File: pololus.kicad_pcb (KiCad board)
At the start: 2 copper layers, 50 x 50 mm, 9 parts

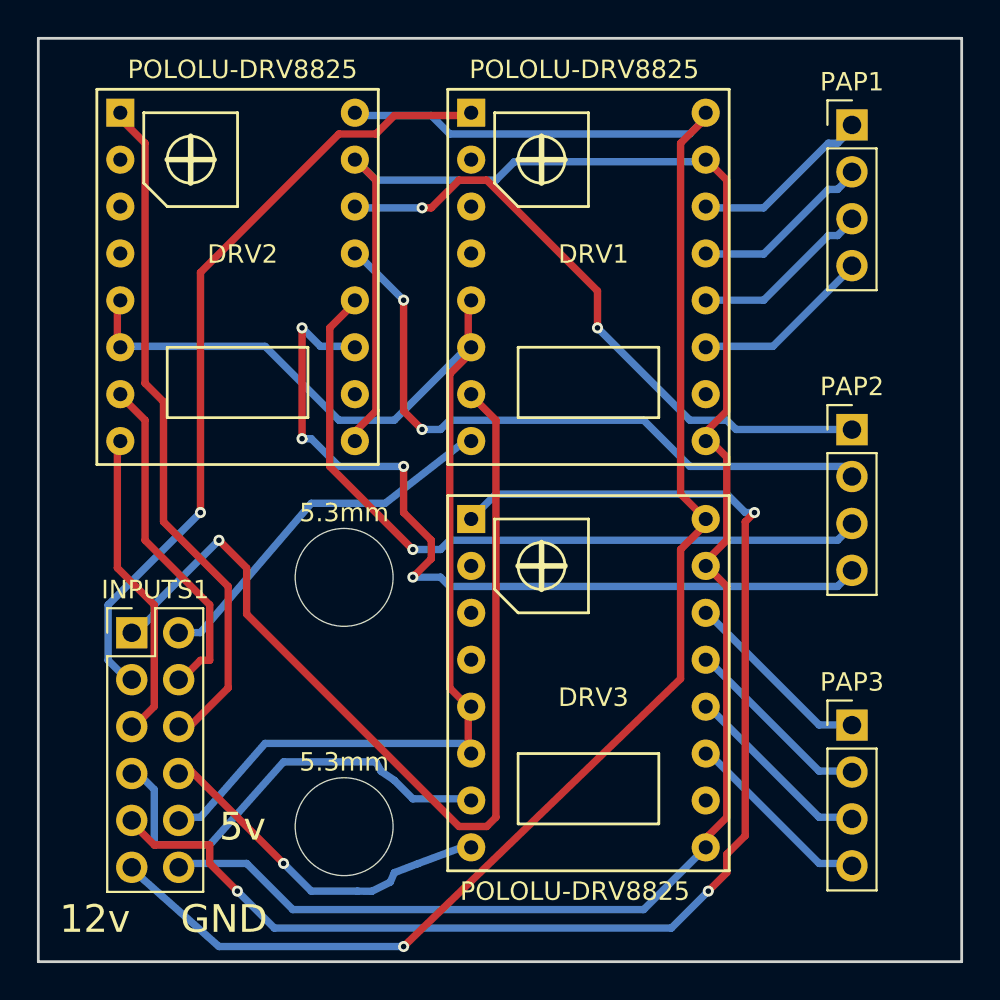
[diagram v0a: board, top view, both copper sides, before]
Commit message: Dev pololus
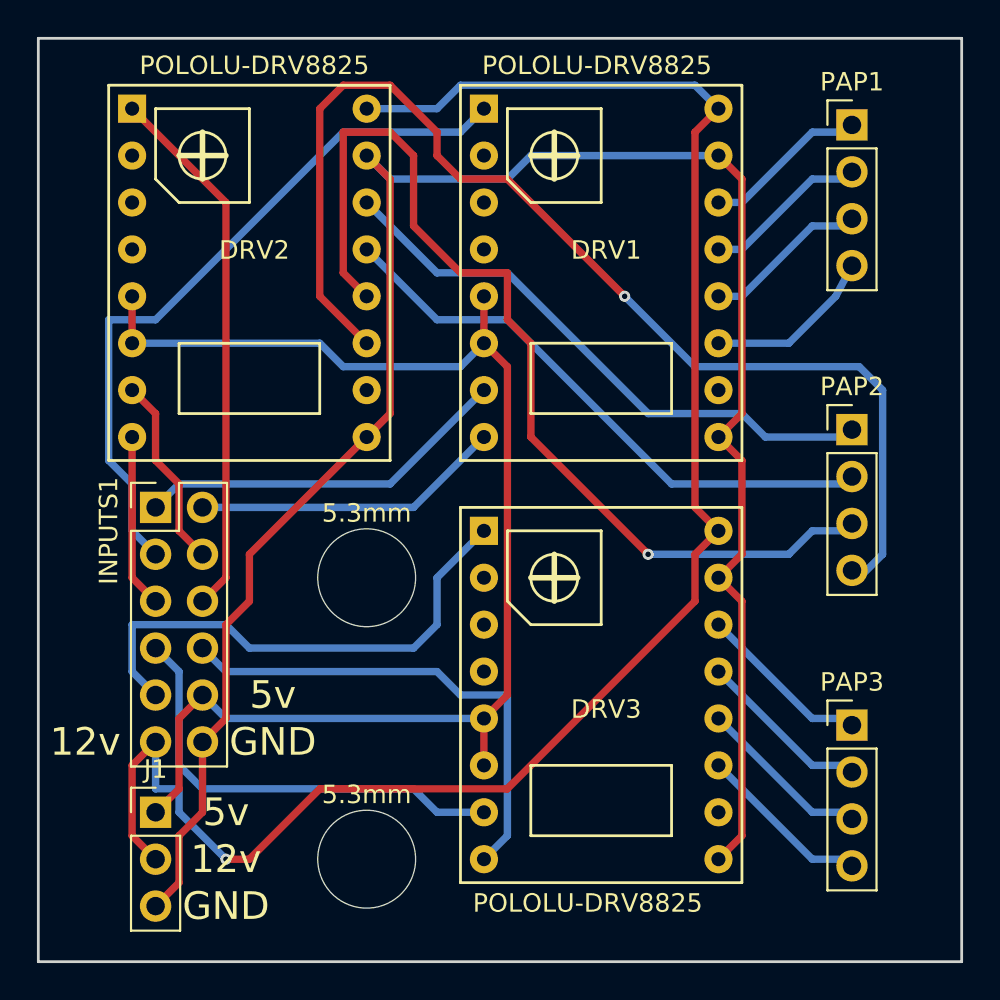
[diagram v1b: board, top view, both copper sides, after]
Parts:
- added J1: Conn_01x03, Pin_Headers:Pin_Header_Straight_1x03_Pitch2.54mm, F.Cu at (115.6, 125.7)
- moved INPUTS1 6.91 mm to (115.6, 109.2)
- moved 5.3mm 2.14 mm to (127.0, 128.3)
- moved 5.3mm 1.22 mm to (127.0, 113.0)
- moved DRV3 0.94 mm to (141.0, 120.7)
- moved DRV1 0.72 mm to (141.0, 97.8)
- moved DRV2 0.68 mm to (121.9, 97.8)
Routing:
- net Net-(DRV3-Pad1): track 73.8 -> 28.0 mm, vias 3 -> 0
- net Net-(DRV1-Pad7): track 54.0 -> 20.4 mm, vias 1 -> 0
- net Net-(DRV2-Pad11): track 47.6 -> 63.6 mm, vias 4 -> 1
- net Net-(DRV2-Pad12): track 41.0 -> 54.6 mm
- net Net-(DRV2-Pad7): track 18.9 -> 10.5 mm
- net Net-(DRV2-Pad1): track 37.2 -> 29.3 mm
- net Net-(DRV2-Pad8): track 17.2 -> 9.42 mm
- net Net-(DRV3-Pad8): track 19.3 -> 27.0 mm, vias 1 -> 0
- net +12V: track 90.9 -> 95.6 mm
- net Net-(DRV1-Pad1): track 43.5 -> 38.8 mm, vias 1 -> 0
- net Net-(DRV2-Pad13): track 36.3 -> 32.5 mm, vias 2 -> 0
- net Net-(DRV1-Pad8): track 20.3 -> 16.8 mm
- net +5V: track 69.5 -> 72.3 mm
- net Net-(DRV2-Pad14): track 34.8 -> 32.5 mm, vias 2 -> 0
- net Net-(DRV1-Pad11): track 10.3 -> 9.28 mm
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
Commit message: Release DLL
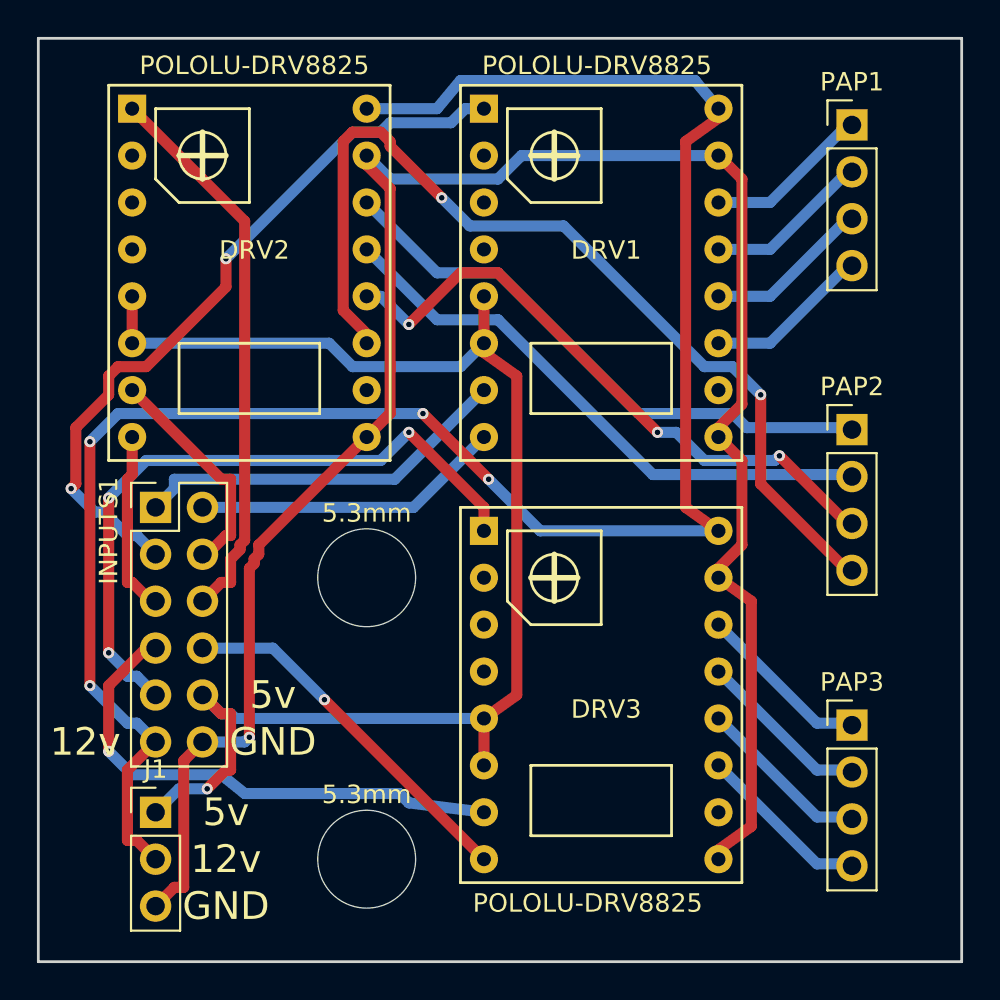
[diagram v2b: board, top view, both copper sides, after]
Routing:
- net Net-(DRV2-Pad12): track 54.6 -> 33.9 mm, vias 1 -> 3
- net +12V: track 95.6 -> 108.4 mm, vias 1 -> 4
- net Net-(DRV2-Pad11): track 63.6 -> 52.0 mm, vias 1 -> 2
- net Net-(DRV3-Pad1): track 28.0 -> 36.8 mm, vias 0 -> 3
- net Net-(DRV3-Pad8): track 27.0 -> 20.0 mm, vias 0 -> 1
- net Net-(DRV3-Pad7): track 24.4 -> 28.4 mm, vias 0 -> 1
- net +5V: track 72.3 -> 75.6 mm, vias 0 -> 1
- net GND: track 107.8 -> 110.2 mm, vias 0 -> 1
- net Net-(DRV2-Pad7): track 10.5 -> 12.3 mm
- net Net-(DRV1-Pad1): track 38.8 -> 40.2 mm, vias 0 -> 2
- net Net-(DRV2-Pad1): track 29.3 -> 30.4 mm
- net Net-(DRV2-Pad13): track 32.5 -> 31.4 mm
- net Net-(DRV2-Pad14): track 32.5 -> 31.4 mm
- net Net-(DRV1-Pad13): track 9.75 -> 8.94 mm
- net Net-(DRV1-Pad14): track 9.75 -> 8.94 mm
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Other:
- net class Default: trace_width 0.4 -> 0.6
